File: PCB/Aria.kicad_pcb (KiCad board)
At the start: 4 copper layers, 30 x 71.5 mm, 86 parts, among them J1 B2B-PH-K-S(LF)(SN), J2 B3B-PH-K-S(LF)(SN), J3 20021121-00010C4LF, J4 0475890001-MicroUSBPort, P1 CONN_01X18, P2 CONN_01X18, Q1 DMG2307L-7, Q2 DMG2307L-7, SW1 B3U-1000P, SW2 B3U-1000P, T1 1909763-1, U1 BQ24210DQCT, U2 AZ1117CR-3.3TRG1_1, U3 STM32F446RET6_-_TQFP64, U4 ESP8285, X1 ABM3B8.000MHZB2T, X2 ABS07-32.768KHZ-9-T, X3 FA-128_26.0000MF10Z-AC3

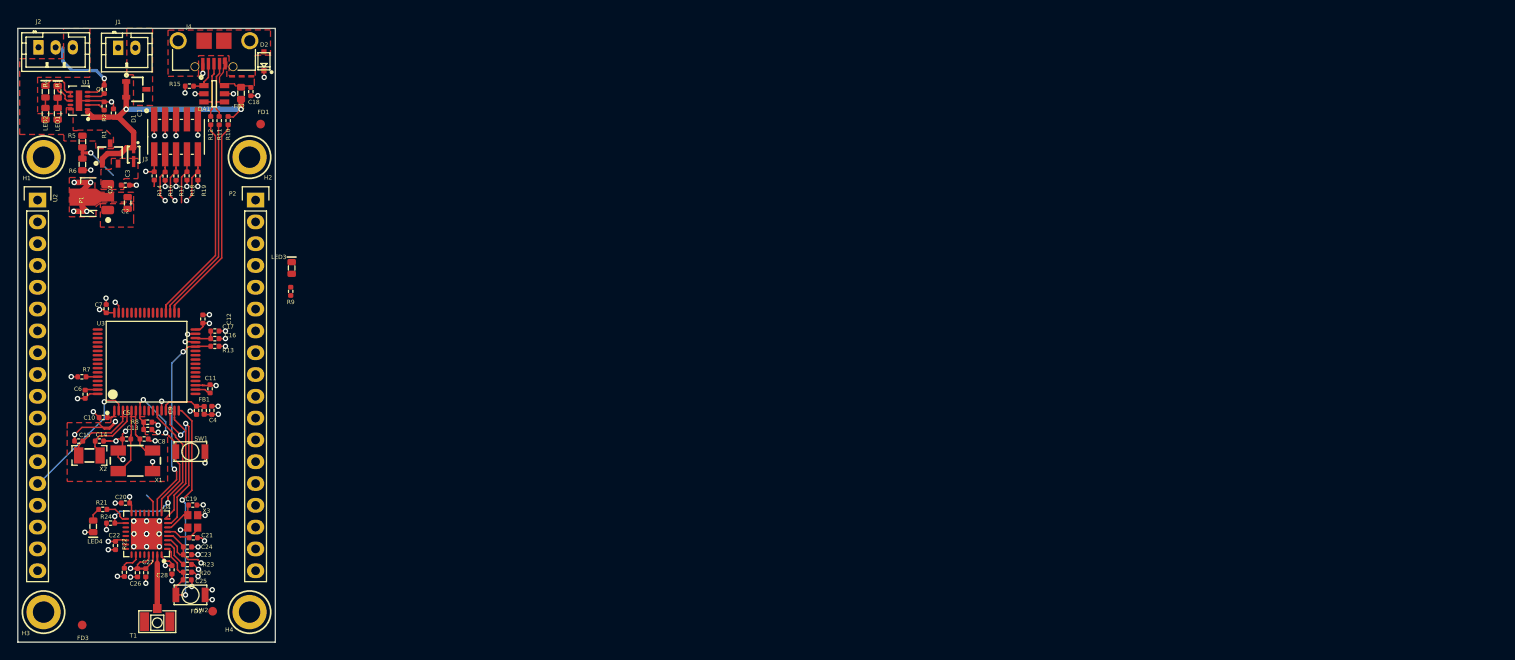
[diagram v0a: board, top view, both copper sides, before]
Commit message: Board Finished
Board finished
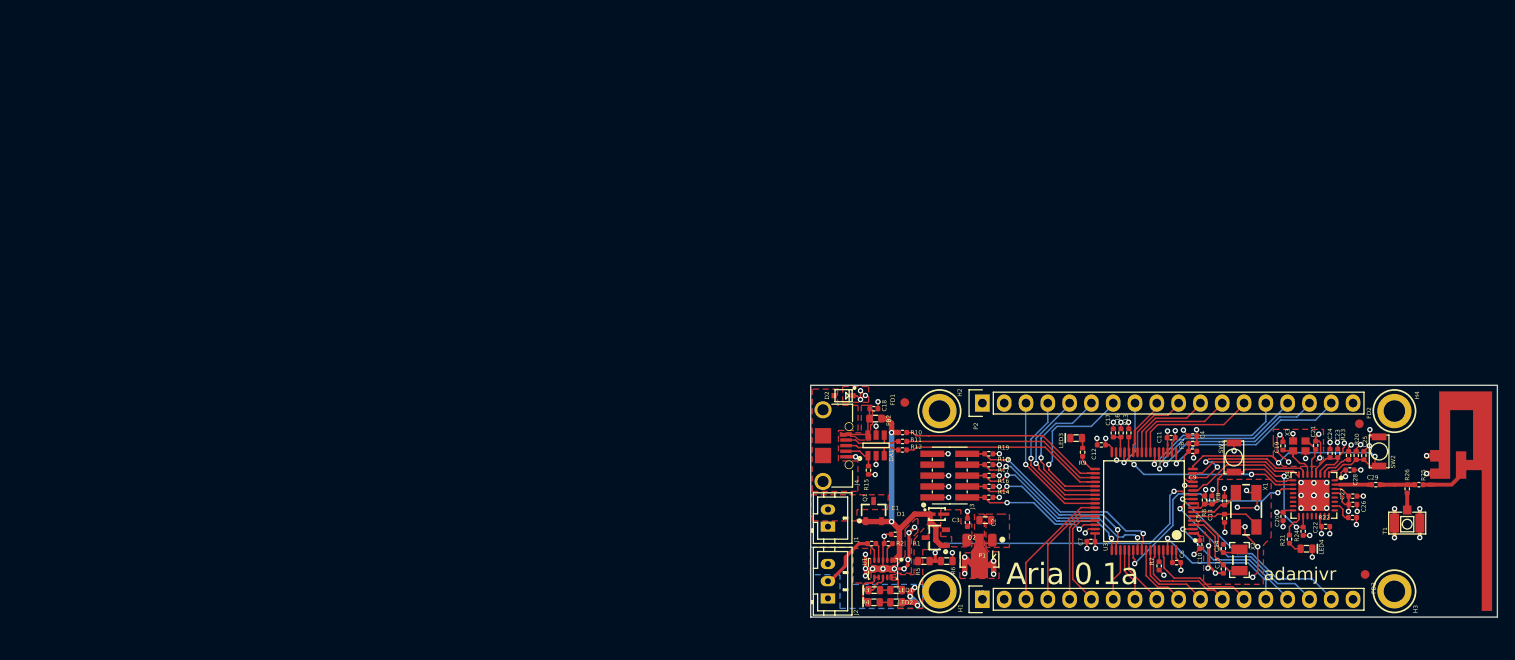
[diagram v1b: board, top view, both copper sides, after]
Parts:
- added ANT1: Inverted_F_PCB_Antenna, PCB_Footprints:PCB_IF_ANT_2.4G, F.Cu at (225.3, 72.3)
- added C29: 600L5R6BT200T, PCB_Footprints:C0402, F.Cu at (211.7, 83.2)
- added R25: ERJ-2GE0R00X, PCB_Footprints:R0402, F.Cu at (216.7, 83.2)
- added R26: ERJ-2GE0R00X, PCB_Footprints:R0402, F.Cu at (215.4, 83.6)
- moved H3 157.4 mm to (213.9, 95.6), turned to 90 degrees
- moved FD3 149.6 mm to (210.5, 93.6), turned to 90 degrees
- moved T1 146.1 mm to (215.4, 87.6)
- moved R22 143.2 mm to (209.0, 87.0), turned to 0 degrees
- moved C26 141.8 mm to (209.0, 85.5), turned to 0 degrees
- moved LED4 141.4 mm to (203.6, 90.6), turned to 0 degrees
- moved C22 141.0 mm to (205.9, 88.0), turned to 0 degrees
- moved C27 140.9 mm to (209.0, 84.5), turned to 0 degrees
- moved SW2 139.5 mm to (212.1, 79.3), turned to 270 degrees
- moved R24 138.9 mm to (203.2, 88.6), turned to 90 degrees
- moved R21 138.3 mm to (201.6, 89.5), turned to 90 degrees
- moved C25 137.8 mm to (210.3, 79.8), turned to 90 degrees
- moved C28 137.7 mm to (208.7, 81.4), turned to 0 degrees
- moved R20 136.8 mm to (209.4, 79.8), turned to 90 degrees
- moved U4 136.1 mm to (204.5, 84.4), turned to 180 degrees
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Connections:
- P1 pad 10: /MCU_STM32F446RET6/PB6 -> /MCU_STM32F446RET6/PB5
- P1 pad 11: /MCU_STM32F446RET6/PB7 -> /MCU_STM32F446RET6/PB6
- P1 pad 12: /MCU_STM32F446RET6/PB8 -> /MCU_STM32F446RET6/PB7
- P1 pad 13: /MCU_STM32F446RET6/PB9 -> /MCU_STM32F446RET6/PB8
- P1 pad 14: /MCU_STM32F446RET6/PC13 -> /MCU_STM32F446RET6/PB9
- P1 pad 15: /MCU_STM32F446RET6/PC0 -> /MCU_STM32F446RET6/PC13
- P1 pad 16: /MCU_STM32F446RET6/PC1 -> /MCU_STM32F446RET6/PC0
- P1 pad 17: /MCU_STM32F446RET6/PC9 -> /MCU_STM32F446RET6/PC1
- P1 pad 3: /MCU_STM32F446RET6/PA10 -> /MCU_STM32F446RET6/PA9
- P1 pad 4: /MCU_STM32F446RET6/PA11 -> /MCU_STM32F446RET6/PA10
- P1 pad 5: /MCU_STM32F446RET6/PA12 -> /MCU_STM32F446RET6/PA11
- P1 pad 6: /MCU_STM32F446RET6/PC10 -> /MCU_STM32F446RET6/PA12
- P1 pad 7: /MCU_STM32F446RET6/PC11 -> /MCU_STM32F446RET6/PC10
- P1 pad 8: /MCU_STM32F446RET6/PC12 -> /MCU_STM32F446RET6/PC11
- P1 pad 9: /MCU_STM32F446RET6/PB5 -> /MCU_STM32F446RET6/PC12
- P2 pad 3: /MCU_STM32F446RET6/PA9 -> /MCU_STM32F446RET6/PA8
- P2 pad 4: /MCU_STM32F446RET6/PA8 -> /MCU_STM32F446RET6/PC9
- T1 pad 1: /WiFi-ESP8285/ANTENNA -> /WiFi-ESP8285/ANT_UM
- U4 pad 2: /WiFi-ESP8285/ANTENNA -> /WiFi-ESP8285/LNA
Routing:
- net GND: track 91.6 -> 131.0 mm, vias 58 -> 82
- net /MCU_STM32F446RET6/BAT_VOLT: track 5.97 -> 37.4 mm, vias 1 -> 2
- net /MCU_STM32F446RET6/ESPTOST_BOOT0: track 1.95 -> 26.2 mm, vias 0 -> 2
- net /MCU_STM32F446RET6/PC1: track 0.00 -> 23.4 mm, vias 0 -> 1
- net /MCU_STM32F446RET6/PA3: track 0.00 -> 22.4 mm, vias 0 -> 1
- net /MCU_STM32F446RET6/PA4: track 0.00 -> 21.3 mm, vias 0 -> 1
- net /MCU_STM32F446RET6/PC0: track 0.00 -> 21.3 mm, vias 0 -> 1
- net /MCU_STM32F446RET6/NJTRST: track 5.49 -> 26.4 mm, vias 0 -> 2
- net /MCU_STM32F446RET6/PA5: track 0.54 -> 21.0 mm, vias 0 -> 1
- net /MCU_STM32F446RET6/PC6: track 0.00 -> 19.4 mm, vias 0 -> 1
- net /MCU_STM32F446RET6/SWO_TDO: track 5.88 -> 25.1 mm, vias 1 -> 2
- net /MCU_STM32F446RET6/PA6: track 0.00 -> 18.6 mm, vias 0 -> 1
- net /MCU_STM32F446RET6/PC7: track 0.00 -> 18.4 mm, vias 0 -> 1
- net /MCU_STM32F446RET6/SWO_TDI: track 5.90 -> 23.5 mm, vias 0 -> 2
- net /MCU_STM32F446RET6/PC8: track 0.00 -> 17.2 mm, vias 0 -> 1
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- added copper zone on B.Cu, net /Power/BAT
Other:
- board size 30 x 71.5 mm -> 80 x 27 mm
- board text added: "Aria 0.1a"
- board text added: "GND 3V3 PA8 PC9 PC8 PC7 PC6 PB10 PB1 PB0 PC5 PC4 PA7 PA6 PA5 PA4 PA3 GND"
- board text added: "GND 3V3 PA9 PA10 PA11 PA12 PC10 PC11 PC12 PB5 PB6 PB7 PB8 PB9 PC13 PC0 PC1 GND"
- board text added: "GND SOLAR V+"
- board text added: "GND THERM BATTERY"
- board text added: "Solar+WiFi Dev Kit https://github.com/adamjvr/Aria"
- board text added: "adamjvr"
